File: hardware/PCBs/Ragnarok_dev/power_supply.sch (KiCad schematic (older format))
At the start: 29 parts, among them Q1 Q_PMOS_GDS, Q2 Q_PMOS_GDS, SW3 Power, U5 TPS62142, U6 RT9069-50GB

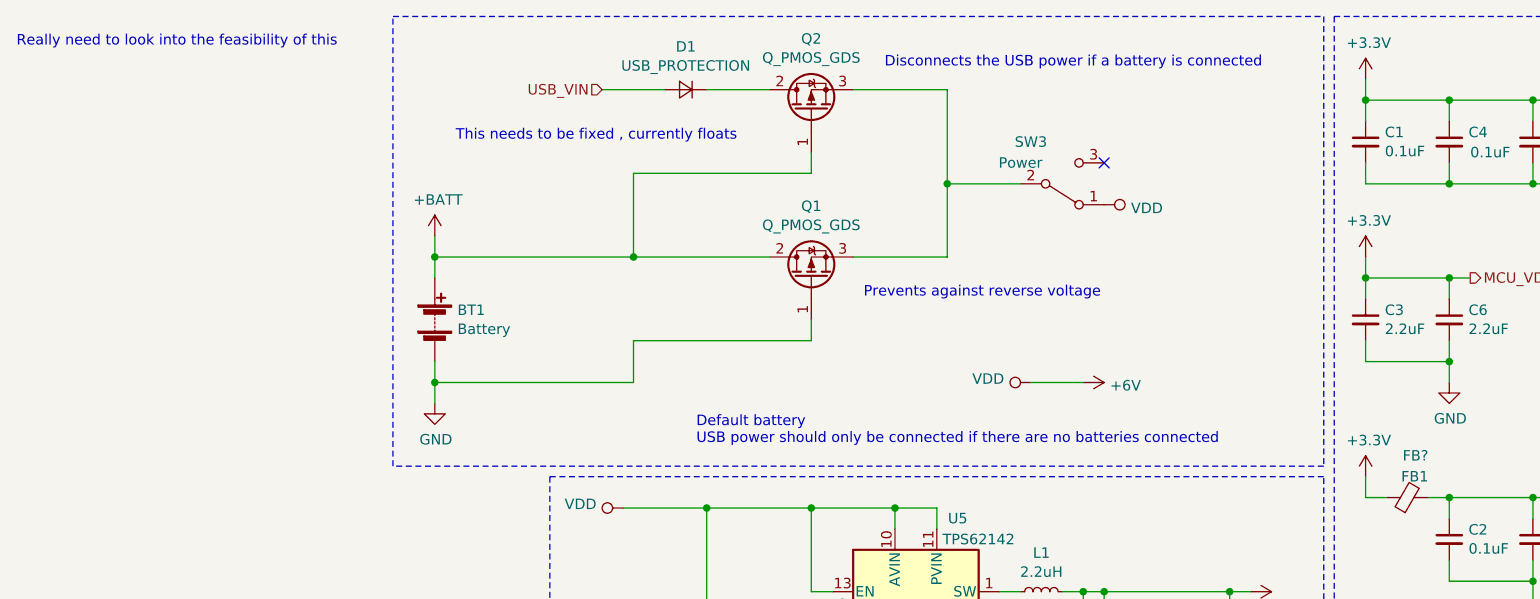
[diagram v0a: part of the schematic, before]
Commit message: update
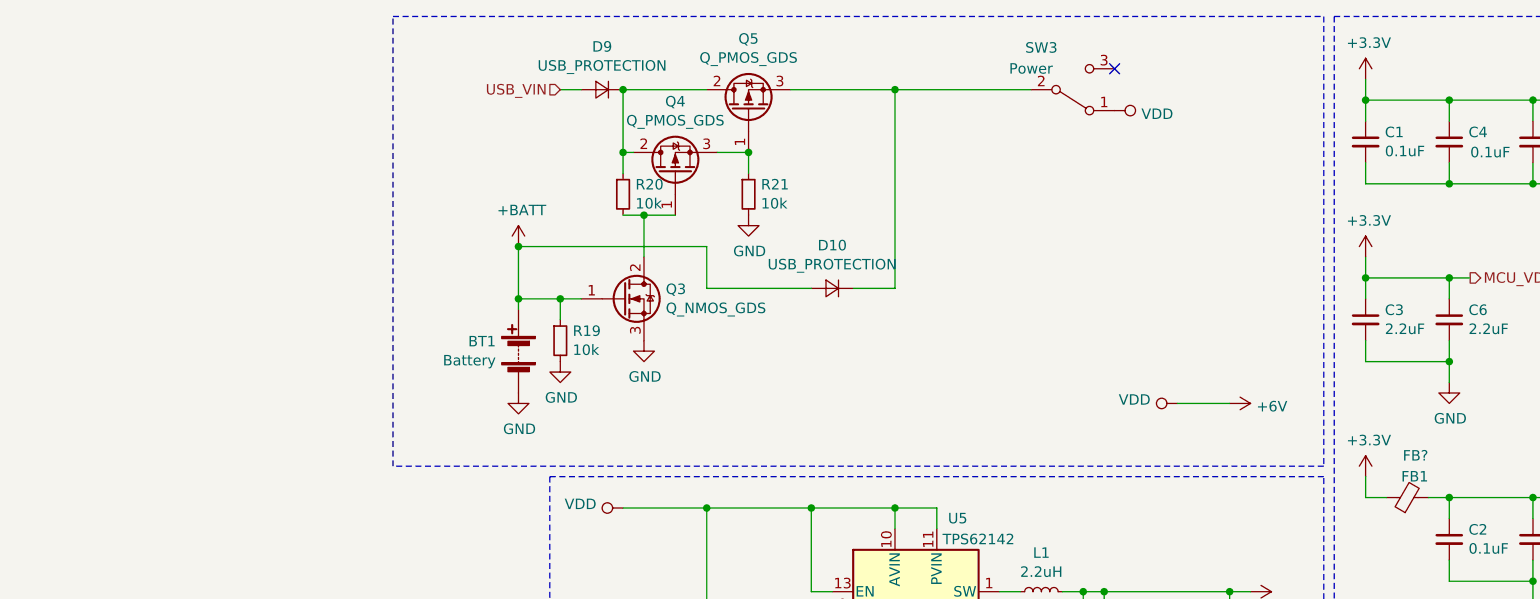
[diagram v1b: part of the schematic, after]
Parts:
- removed D1: USB_PROTECTION, symbol Device:D_Small
- removed Q1, Q2: Q_PMOS_GDS, Package_TO_SOT_SMD:SOT-223-3_TabPin2, symbol Device:Q_PMOS_GDS
- added D10, D9: USB_PROTECTION, Diode_SMD:D_0603_1608Metric_Pad1.05x0.95mm_HandSolder, symbol Device:D_Small
- added Q3: Q_NMOS_GDS, symbol Device:Q_NMOS_GDS
- added Q4, Q5: Q_PMOS_GDS, Package_TO_SOT_SMD:SOT-223-3_TabPin2, symbol Device:Q_PMOS_GDS
- added R19, R20, R21: 10k, Resistor_SMD:R_0603_1608Metric_Pad1.05x0.95mm_HandSolder, symbol Device:R_Small
- BT1: footprint (none) -> Connector_JST:JST_GH_SM02B-GHS-TB_1x02-1MP_P1.25mm_Horizontal
- C24, C25: footprint (none) -> Capacitor_SMD:C_0603_1608Metric_Pad1.05x0.95mm_HandSolder
- FB1, L1: footprint (none) -> Inductor_SMD:L_0603_1608Metric_Pad1.05x0.95mm_HandSolder
- R3: footprint (none) -> Resistor_SMD:R_0603_1608Metric_Pad1.05x0.95mm_HandSolder
- U6: footprint (none) -> Package_TO_SOT_SMD:SOT-23-5
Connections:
- net +BATT: now also D10.2 (A), Q3.1 (G), R19.1
- net GND: now also Q3.3 (S), R19.2, R21.2
- net USB_VIN: now also D9.2 (A)
- net at SW3.2 (B): now also D10.1 (K), Q5.3 (S)
- new net: Q4.3 (S), Q5.1 (G), R21.1
- new net: D9.1 (K), Q4.2 (D), Q5.2 (D), R20.1
- new net: Q3.2 (D), Q4.1 (G), R20.2
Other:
- note removed: "Default battery\nUSB power should only be connected if there are no batteries connected"
- note removed: "Disconnects the USB power if a battery is connected"
- note removed: "Prevents against reverse voltage"
- note removed: "Really need to look into the feasibility of this"
- note removed: "This needs to be fixed , currently floats\n"
